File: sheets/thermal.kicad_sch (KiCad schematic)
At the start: 0 parts

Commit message: pushing storage
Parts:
- added U1, U3, U4, U5, U6, U7, U8, U9: MAX31856, Package_SO:TSSOP-14_4.4x5mm_P0.65mm, symbol Sensor_Temperature:MAX31856

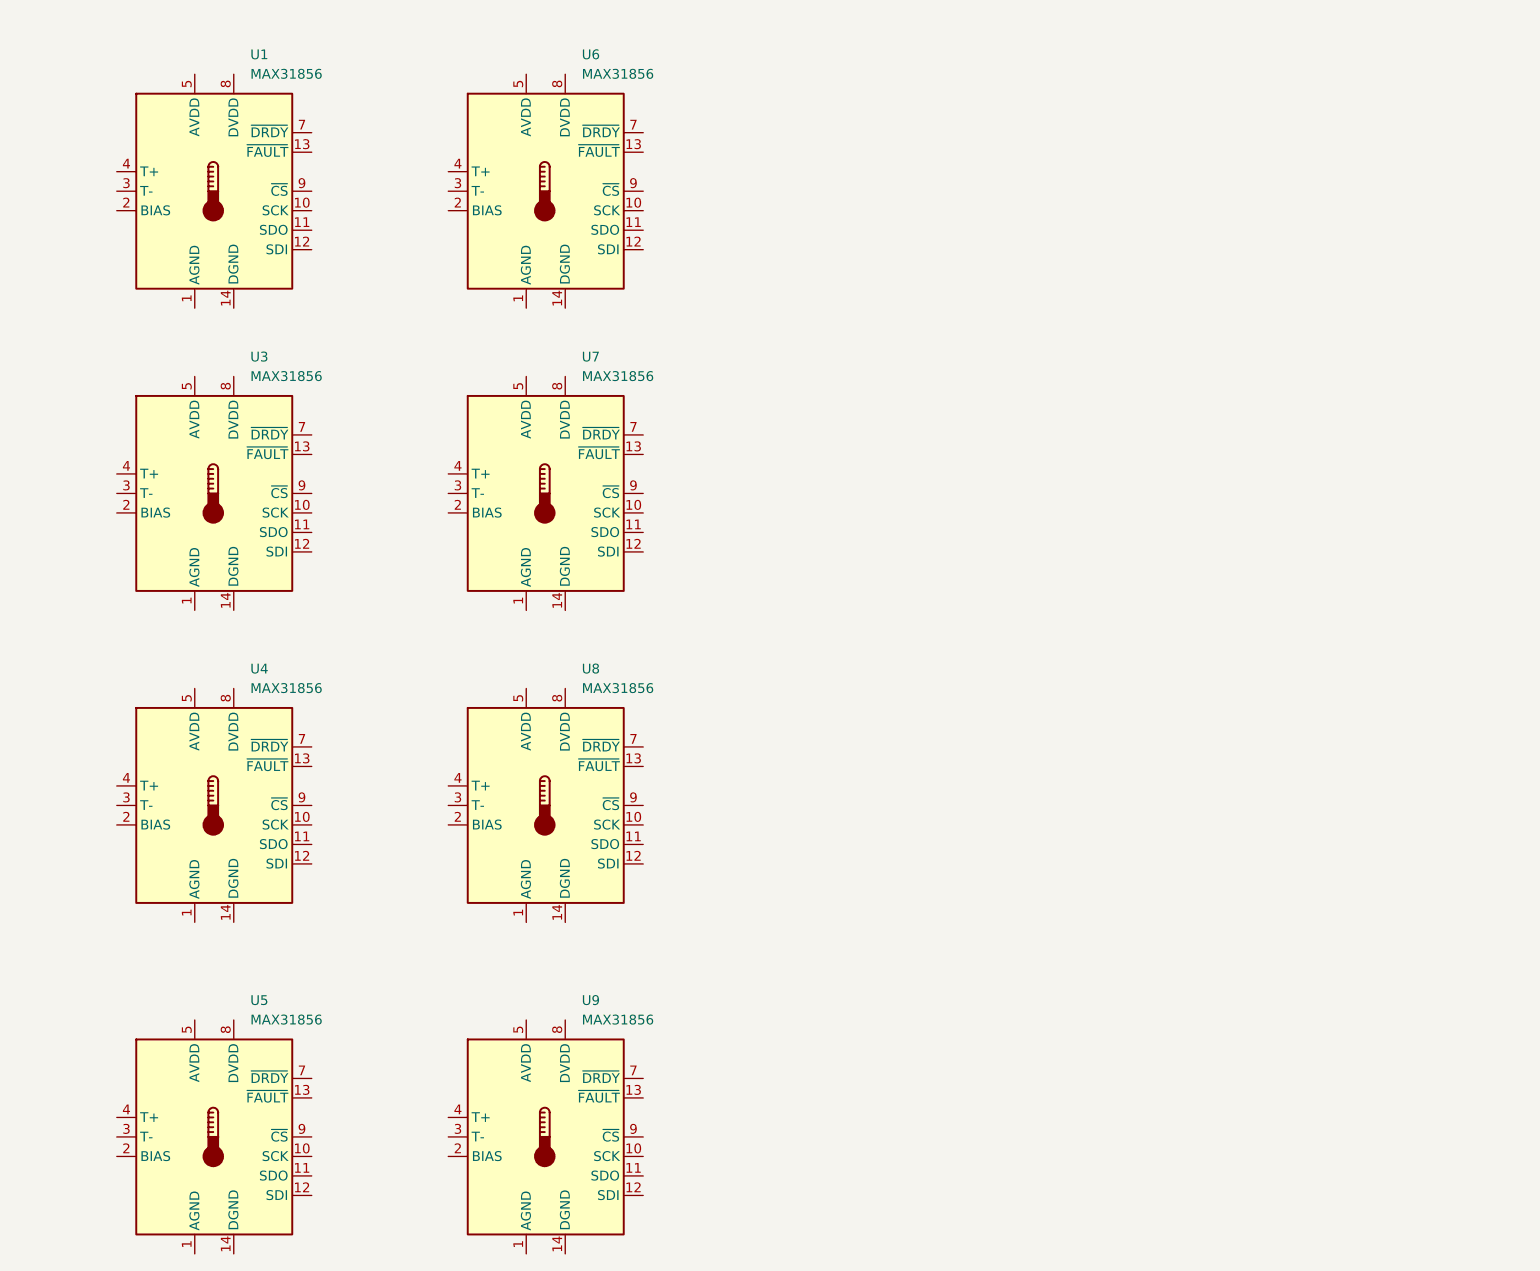
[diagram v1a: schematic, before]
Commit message: push
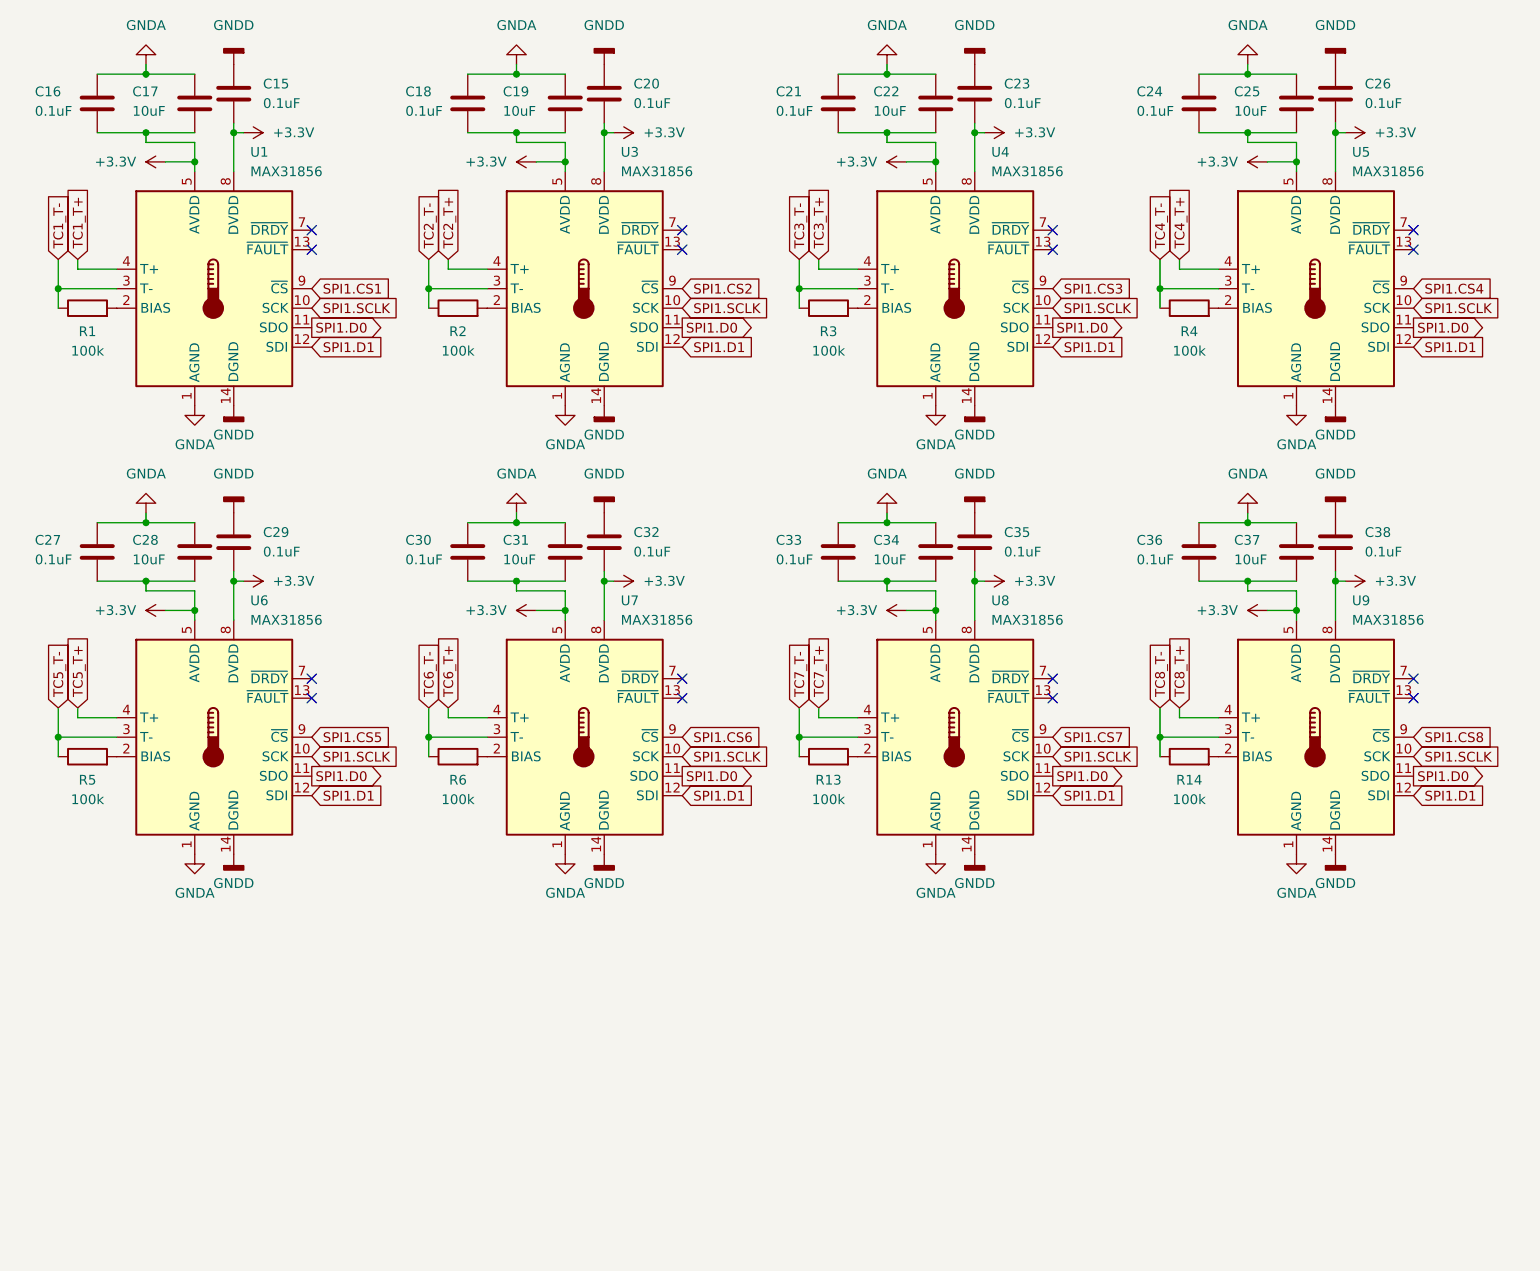
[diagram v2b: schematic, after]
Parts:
- added C15, C16, C18, C20, C21, C23, C24, C26, C27, C29, C30, C32, C33, C35, C36, C38: 0.1uF, symbol Device:C
- added C17, C19, C22, C25, C28, C31, C34, C37: 10uF, symbol Device:C
- added R1, R13, R14, R2, R3, R4, R5, R6: 100k, symbol Device:R
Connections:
- net GNDA: now reaches U8.1 (AGND)
- net GNDA: now also U1.1 (AGND), U3.1 (AGND), U4.1 (AGND), U5.1 (AGND), U6.1 (AGND), U7.1 (AGND), U9.1 (AGND), C16.1, C17.1, C18.1, C19.1, C21.1, C22.1, C24.1, C25.1, C27.1, C28.1, C30.1, C31.1, C33.1, C34.1, C36.1, C37.1
- net SPI1.SCLK: now reaches U8.10 (SCK)
- net SPI1.SCLK: now also U1.10 (SCK), U3.10 (SCK), U4.10 (SCK), U5.10 (SCK), U6.10 (SCK), U7.10 (SCK), U9.10 (SCK)
- net SPI1.D0: now reaches U8.11 (SDO)
- net SPI1.D0: now also U1.11 (SDO), U3.11 (SDO), U4.11 (SDO), U5.11 (SDO), U6.11 (SDO), U7.11 (SDO), U9.11 (SDO)
- net SPI1.D1: now reaches U8.12 (SDI)
- net SPI1.D1: now also U1.12 (SDI), U3.12 (SDI), U4.12 (SDI), U5.12 (SDI), U6.12 (SDI), U7.12 (SDI), U9.12 (SDI)
- net GNDD: now reaches U8.14 (DGND)
- net GNDD: now also U1.14 (DGND), U3.14 (DGND), U4.14 (DGND), U5.14 (DGND), U6.14 (DGND), U7.14 (DGND), U9.14 (DGND), C15.1, C20.1, C23.1, C26.1, C29.1, C32.1, C35.1, C38.1
- net at U8.2 (BIAS): now also R13.2
- net TC7_T-: now reaches U8.3 (T-)
- net TC7_T-: now also R13.1
- net TC7_T+: now reaches U8.4 (T+)
- net +3.3V: now reaches U8.5 (AVDD)
- net +3.3V: now also U1.5 (AVDD), U1.8 (DVDD), U3.5 (AVDD), U3.8 (DVDD), U4.5 (AVDD), U4.8 (DVDD), U5.5 (AVDD), U5.8 (DVDD), U6.5 (AVDD), U6.8 (DVDD), U7.5 (AVDD), U7.8 (DVDD), U8.8 (DVDD), U9.5 (AVDD), U9.8 (DVDD), C15.2, C16.2, C17.2, C18.2, C19.2, C20.2, C21.2, C22.2, C23.2, C24.2, C25.2, C26.2, C27.2, C28.2, C29.2, C30.2, C31.2, C32.2, C33.2, C34.2, C35.2, C36.2, C37.2, C38.2
- net SPI1.CS7: now reaches U8.9 (~{CS})
- net at U4.2 (BIAS): now also R3.2
- net TC3_T-: now reaches U4.3 (T-)
- net TC3_T-: now also R3.1
- net TC3_T+: now reaches U4.4 (T+)
- net SPI1.CS3: now reaches U4.9 (~{CS})
- net at U9.2 (BIAS): now also R14.2
- net TC8_T-: now reaches U9.3 (T-)
- net TC8_T-: now also R14.1
- net TC8_T+: now reaches U9.4 (T+)
- net SPI1.CS8: now reaches U9.9 (~{CS})
- net at U7.2 (BIAS): now also R6.2
- net TC6_T-: now reaches U7.3 (T-)
- net TC6_T-: now also R6.1
- net TC6_T+: now reaches U7.4 (T+)
- net SPI1.CS6: now reaches U7.9 (~{CS})
- net at U3.2 (BIAS): now also R2.2
- net TC2_T-: now reaches U3.3 (T-)
- net TC2_T-: now also R2.1
- net TC2_T+: now reaches U3.4 (T+)
- net SPI1.CS2: now reaches U3.9 (~{CS})
- net at U1.2 (BIAS): now also R1.2
- net TC1_T-: now reaches U1.3 (T-)
- net TC1_T-: now also R1.1
- net TC1_T+: now reaches U1.4 (T+)
- net SPI1.CS1: now reaches U1.9 (~{CS})
- net at U5.2 (BIAS): now also R4.2
- net TC4_T-: now reaches U5.3 (T-)
- net TC4_T-: now also R4.1
- net TC4_T+: now reaches U5.4 (T+)
- net SPI1.CS4: now reaches U5.9 (~{CS})
- net at U6.2 (BIAS): now also R5.2
- net TC5_T-: now reaches U6.3 (T-)
- net TC5_T-: now also R5.1
- net TC5_T+: now reaches U6.4 (T+)
- net SPI1.CS5: now reaches U6.9 (~{CS})
- no-connect marks 0 -> 16
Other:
- moved on the sheet: U1

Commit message: allocating pins ?
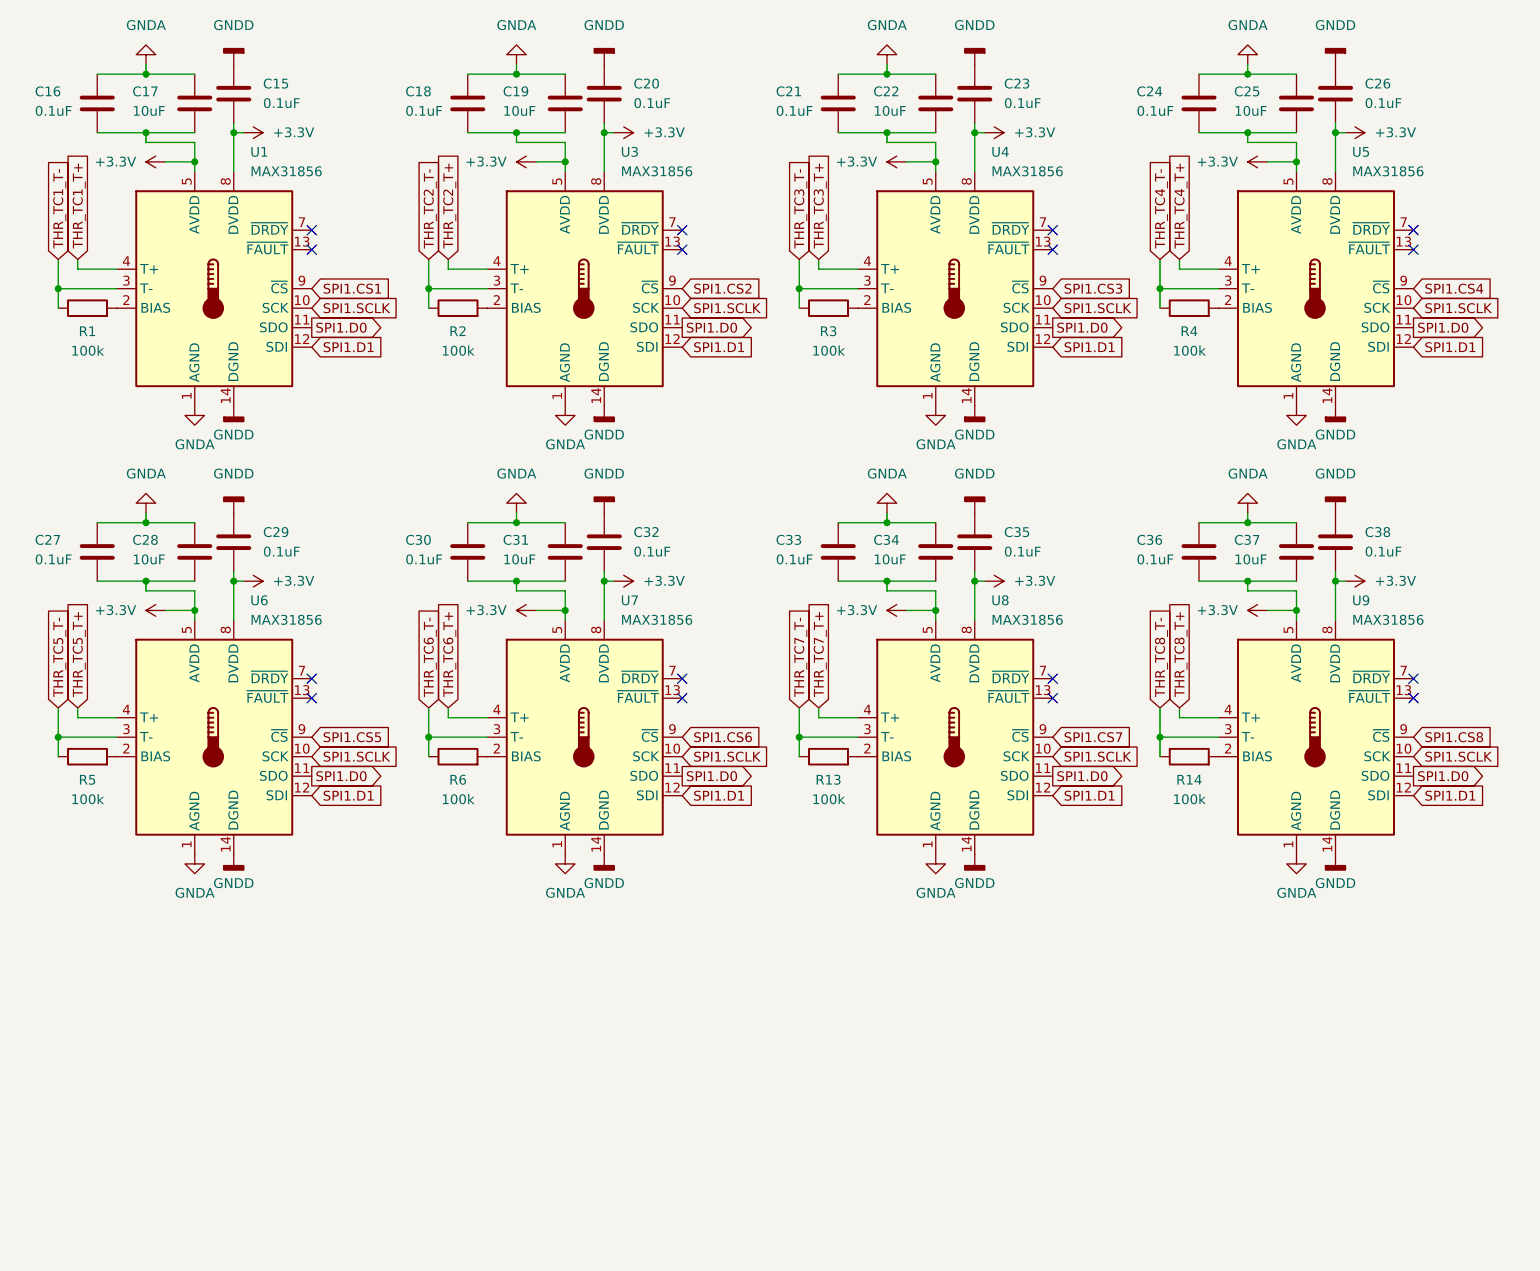
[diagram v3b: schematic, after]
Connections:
- net TC1_T+ renamed THR_TC1_T+
- net TC1_T- renamed THR_TC1_T-
- net TC2_T+ renamed THR_TC2_T+
- net TC2_T- renamed THR_TC2_T-
- net TC3_T+ renamed THR_TC3_T+
- net TC3_T- renamed THR_TC3_T-
- net TC4_T+ renamed THR_TC4_T+
- net TC4_T- renamed THR_TC4_T-
- net TC5_T+ renamed THR_TC5_T+
- net TC5_T- renamed THR_TC5_T-
- net TC6_T+ renamed THR_TC6_T+
- net TC6_T- renamed THR_TC6_T-
- net TC7_T+ renamed THR_TC7_T+
- net TC7_T- renamed THR_TC7_T-
- net TC8_T+ renamed THR_TC8_T+
- net TC8_T- renamed THR_TC8_T-
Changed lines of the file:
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@@
 		)
 	)
-	(global_label "TC2_T+"
+	(global_label "THR_TC2_T+"
 		(shape input)
 		(at 69.85 45.72 90)
@@
 		)
 		(property "Intersheetrefs" "${INTERSHEET_REFS}"
-			(at 69.85 35.685 90)
-			(hide yes)
-			(show_name no)
-			(do_not_autoplace no)
-			(effects
-				(font
-					(size 1.27 1.27)
-				)
-				(justify left)
-			)
-		)
-	)
-	(global_label "TC5_T+"
+			(at 69.85 31.1493 90)
+			(hide yes)
+			(show_name no)
+			(do_not_autoplace no)
+			(effects
+				(font
+					(size 1.27 1.27)
+				)
+				(justify left)
+			)
+		)
+	)
+	(global_label "THR_TC5_T+"
 		(shape input)
 		(at 21.59 104.14 90)
@@
 		)
 		(property "Intersheetrefs" "${INTERSHEET_REFS}"
-			(at 21.59 94.105 90)
-			(hide yes)
-			(show_name no)
-			(do_not_autoplace no)
-			(effects
-				(font
-					(size 1.27 1.27)
-				)
-				(justify left)
-			)
-		)
-	)
-	(global_label "TC5_T-"
+			(at 21.59 89.5693 90)
+			(hide yes)
+			(show_name no)
+			(do_not_autoplace no)
+			(effects
+				(font
+					(size 1.27 1.27)
+				)
+				(justify left)
+			)
+		)
+	)
+	(global_label "THR_TC5_T-"
 		(shape input)
 		(at 19.05 104.14 90)
@@
 		)
 		(property "Intersheetrefs" "${INTERSHEET_REFS}"
-			(at 19.05 94.105 90)
+			(at 19.05 89.5693 90)
 			(hide yes)
 			(show_name no)
@@
 		)
 	)
-	(global_label "TC4_T+"
+	(global_label "THR_TC4_T+"
 		(shape input)
 		(at 165.1 45.72 90)
@@
 		)
 		(property "Intersheetrefs" "${INTERSHEET_REFS}"
-			(at 165.1 35.685 90)
+			(at 165.1 31.1493 90)
 			(hide yes)
 			(show_name no)
@@
 		)
 	)
-	(global_label "TC6_T+"
+	(global_label "THR_TC6_T+"
 		(shape input)
 		(at 69.85 104.14 90)
@@
 		)
 		(property "Intersheetrefs" "${INTERSHEET_REFS}"
-			(at 69.85 94.105 90)
+			(at 69.85 89.5693 90)
 			(hide yes)
 			(show_name no)
@@
 		)
 	)
-	(global_label "TC8_T-"
+	(global_label "THR_TC8_T-"
 		(shape input)
 		(at 162.56 104.14 90)
@@
 		)
 		(property "Intersheetrefs" "${INTERSHEET_REFS}"
-			(at 162.56 94.105 90)
+			(at 162.56 89.5693 90)
 			(hide yes)
 			(show_name no)
@@
 		)
 	)
-	(global_label "TC3_T+"
+	(global_label "THR_TC3_T+"
 		(shape input)
 		(at 118.11 45.72 90)
@@
 		)
 		(property "Intersheetrefs" "${INTERSHEET_REFS}"
-			(at 118.11 35.685 90)
+			(at 118.11 31.1493 90)
 			(hide yes)
 			(show_name no)
@@
 		)
 	)
-	(global_label "TC1_T-"
+	(global_label "THR_TC1_T-"
 		(shape input)
 		(at 19.05 45.72 90)
@@
 		)
 		(property "Intersheetrefs" "${INTERSHEET_REFS}"
-			(at 19.05 35.685 90)
+			(at 19.05 31.1493 90)
 			(hide yes)
 			(show_name no)
@@
 		)
 	)
-	(global_label "TC2_T-"
+	(global_label "THR_TC2_T-"
 		(shape input)
 		(at 67.31 45.72 90)
@@
 		)
 		(property "Intersheetrefs" "${INTERSHEET_REFS}"
-			(at 67.31 35.685 90)
+			(at 67.31 31.1493 90)
 			(hide yes)
 			(show_name no)
@@
 		)
 	)
-	(global_label "TC7_T+"
+	(global_label "THR_TC7_T+"
 		(shape input)
 		(at 118.11 104.14 90)
@@
 		)
 		(property "Intersheetrefs" "${INTERSHEET_REFS}"
-			(at 118.11 94.105 90)
+			(at 118.11 89.5693 90)
 			(hide yes)
 			(show_name no)
@@
 		)
 	)
-	(global_label "TC8_T+"
+	(global_label "THR_TC8_T+"
 		(shape input)
 		(at 165.1 104.14 90)
@@
 		)
 		(property "Intersheetrefs" "${INTERSHEET_REFS}"
-			(at 165.1 94.105 90)
+			(at 165.1 89.5693 90)
 			(hide yes)
 			(show_name no)
@@
 		)
 	)
-	(global_label "TC7_T-"
+	(global_label "THR_TC7_T-"
 		(shape input)
 		(at 115.57 104.14 90)
@@
 		)
 		(property "Intersheetrefs" "${INTERSHEET_REFS}"
-			(at 115.57 94.105 90)
-			(hide yes)
-			(show_name no)
-			(do_not_autoplace no)
-			(effects
-				(font
-					(size 1.27 1.27)
-				)
-				(justify left)
-			)
-		)
-	)
-	(global_label "TC6_T-"
+			(at 115.57 89.5693 90)
+			(hide yes)
+			(show_name no)
+			(do_not_autoplace no)
+			(effects
+				(font
+					(size 1.27 1.27)
+				)
+				(justify left)
+			)
+		)
+	)
+	(global_label "THR_TC6_T-"
 		(shape input)
 		(at 67.31 104.14 90)
@@
 		)
 		(property "Intersheetrefs" "${INTERSHEET_REFS}"
-			(at 67.31 94.105 90)
+			(at 67.31 89.5693 90)
 			(hide yes)
 			(show_name no)
@@
 		)
 	)
-	(global_label "TC1_T+"
+	(global_label "THR_TC1_T+"
 		(shape input)
 		(at 21.59 45.72 90)
@@
 		)
 		(property "Intersheetrefs" "${INTERSHEET_REFS}"
-			(at 21.59 35.685 90)
+			(at 21.59 31.1493 90)
 			(hide yes)
 			(show_name no)
@@
 		)
 	)
-	(global_label "TC4_T-"
+	(global_label "THR_TC4_T-"
 		(shape input)
 		(at 162.56 45.72 90)
@@
 		)
 		(property "Intersheetrefs" "${INTERSHEET_REFS}"
-			(at 162.56 35.685 90)
+			(at 162.56 31.1493 90)
 			(hide yes)
 			(show_name no)
@@
 		)
 	)
-	(global_label "TC3_T-"
+	(global_label "THR_TC3_T-"
 		(shape input)
 		(at 115.57 45.72 90)
@@
 		)
 		(property "Intersheetrefs" "${INTERSHEET_REFS}"
-			(at 115.57 35.685 90)
-			(hide yes)
-			(show_name no)
+			(at 115.57 31.1493 90)
+			(hide yes)
+			(show_name no)
